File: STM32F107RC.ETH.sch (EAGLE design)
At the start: 28 parts, among them J1 HR911105A, Q1 8MHz, U1 LAN8720A-CP, U2 STM32F107RCT6, X1 CB3LV-3I-74M2500

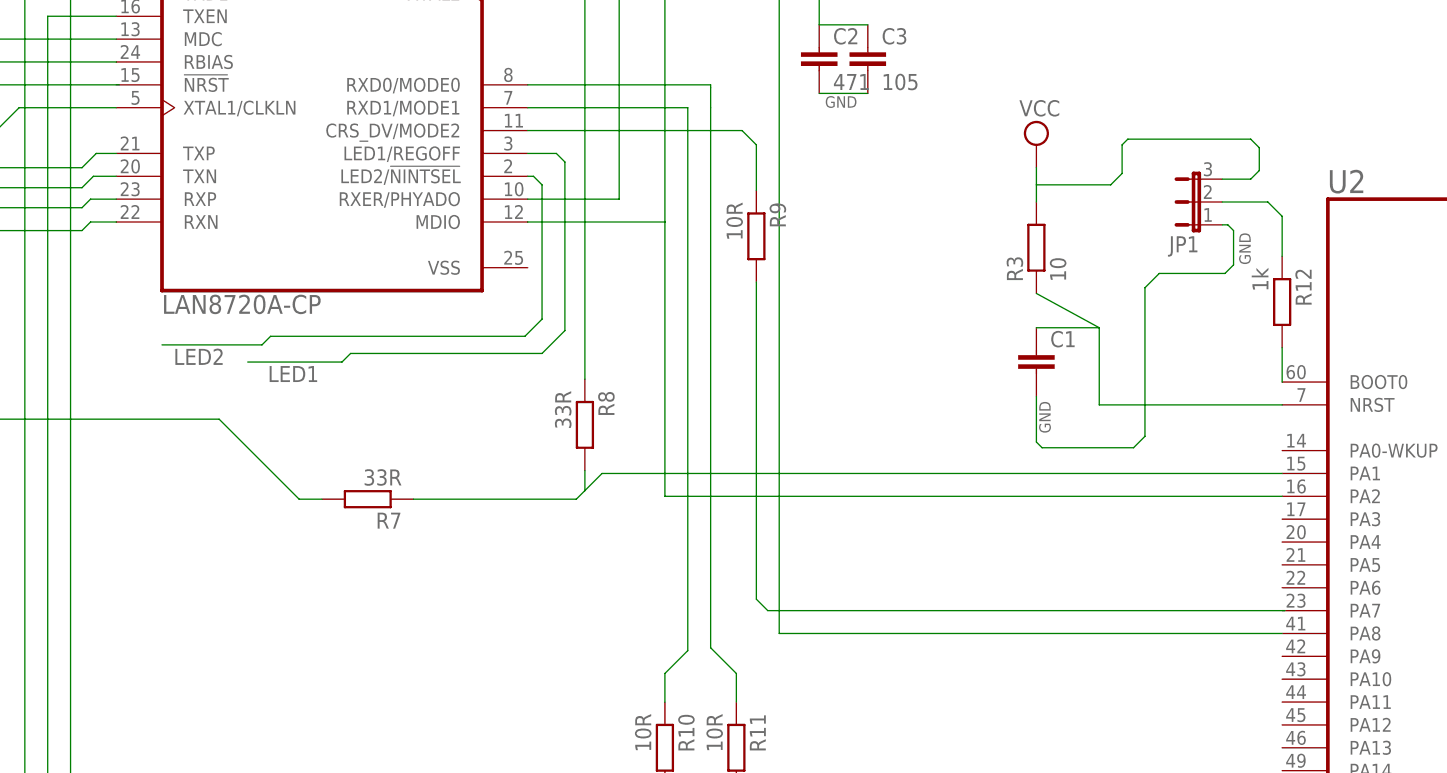
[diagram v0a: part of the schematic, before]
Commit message: Add files via upload
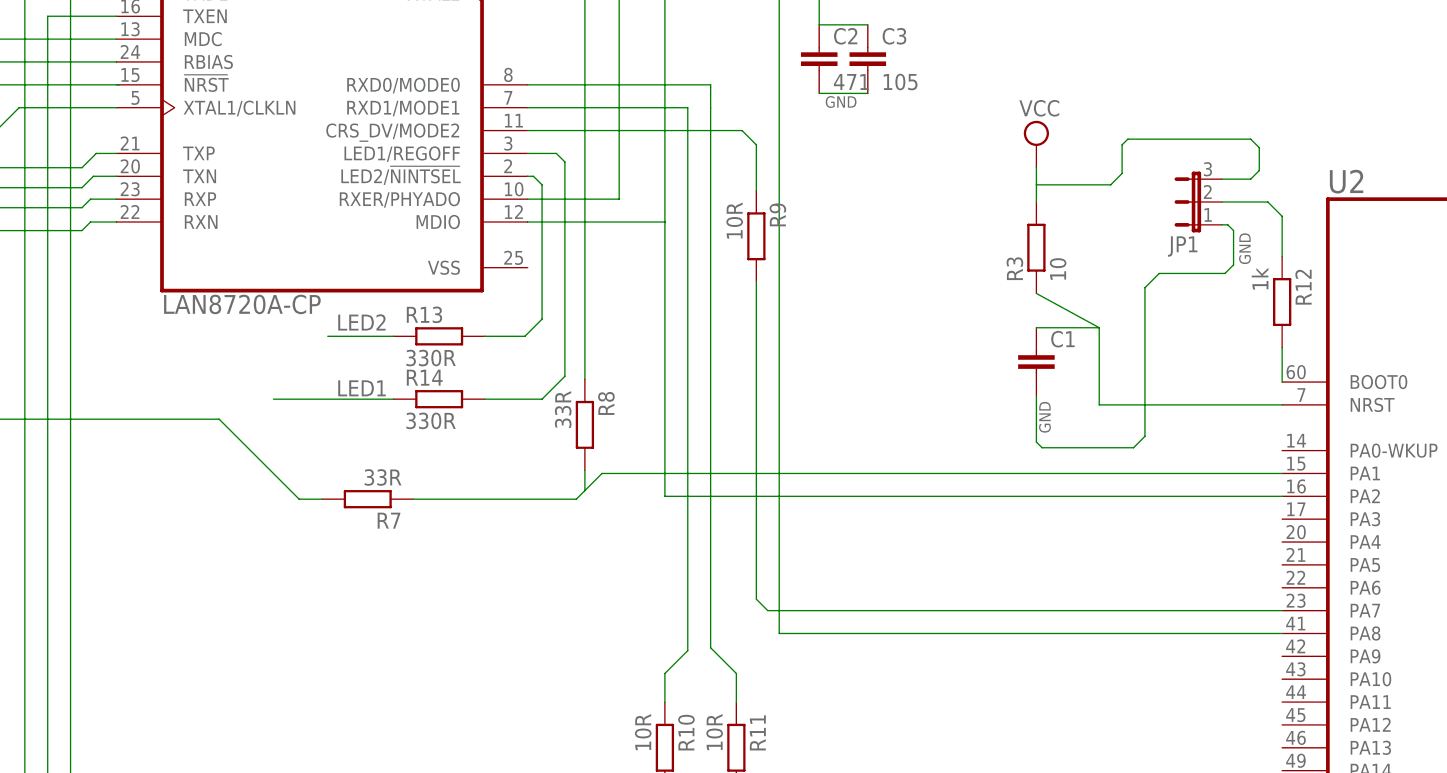
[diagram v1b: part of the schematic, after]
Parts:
- added R13, R14: 330R, resistor:R-EU_0204_7
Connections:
- new net SIG_LED01: R14.2, U1.LED1/REGOFF
- new net SIG_LED02: R13.2, U1.LED2/!NINTSEL!
- net LED1: now also R14.1; no longer U1.LED1/REGOFF
- net LED2: now also R13.1; no longer U1.LED2/!NINTSEL!
- net N$4: now also U2.PA7
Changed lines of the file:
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@@
 <part name="J1" library="HR911105A" deviceset="HR911105A" device=""/>
 <part name="J2" library="SparkFun-Connectors" deviceset="M01" device="OFFSET"/>
+<part name="R13" library="resistor" deviceset="R-EU_" device="0204_7" value="330R"/>
+<part name="R14" library="resistor" deviceset="R-EU_" device="0204_7" value="330R"/>
 </parts>
 <sheets>
@@
 <instance part="J1" gate="G$1" x="-158.115" y="139.3825" rot="R180"/>
 <instance part="J2" gate="G$1" x="17.78" y="198.12" rot="R270"/>
+<instance part="R13" gate="G$1" x="-12.3825" y="124.46"/>
+<instance part="R14" gate="G$1" x="-12.3825" y="117.475"/>
 </instances>
 <busses>
@@
 <net name="N$4" class="0">
 <segment>
-<wire x1="81.5975" y1="93.98" x2="24.13" y2="93.98" width="0.1524" layer="91"/>
+<wire x1="81.28" y1="93.98" x2="24.13" y2="93.98" width="0.1524" layer="91"/>
 <pinref part="R9" gate="G$1" pin="2"/>
 <wire x1="22.86" y1="130.4925" x2="22.86" y2="95.25" width="0.1524" layer="91"/>
 <wire x1="22.86" y1="95.25" x2="24.13" y2="93.98" width="0.1524" layer="91"/>
+<pinref part="U2" gate="A" pin="PA7"/>
 </segment>
 </net>
@@
 <net name="LED2" class="0">
 <segment>
-<pinref part="U1" gate="G$1" pin="LED2/!NINTSEL!"/>
-<wire x1="-2.54" y1="142.24" x2="-1.905" y2="142.24" width="0.1524" layer="91"/>
-<wire x1="-1.905" y1="142.24" x2="-0.9525" y2="141.2875" width="0.1524" layer="91"/>
-<wire x1="-0.9525" y1="141.2875" x2="-0.9525" y2="126.365" width="0.1524" layer="91"/>
-<wire x1="-0.9525" y1="126.365" x2="-2.8575" y2="124.46" width="0.1524" layer="91"/>
-<wire x1="-2.8575" y1="124.46" x2="-31.115" y2="124.46" width="0.1524" layer="91"/>
-<wire x1="-31.115" y1="124.46" x2="-32.0675" y2="123.5075" width="0.1524" layer="91"/>
-<wire x1="-32.0675" y1="123.5075" x2="-43.18" y2="123.5075" width="0.1524" layer="91"/>
-<label x="-41.91" y="121.285" size="1.778" layer="95"/>
-</segment>
-<segment>
 <pinref part="J1" gate="G$1" pin="YC"/>
 <wire x1="-120.015" y1="167.3225" x2="-119.0625" y2="167.3225" width="0.1524" layer="91"/>
@@
 <label x="-118.4275" y="180.975" size="1.778" layer="95" rot="R90"/>
 </segment>
+<segment>
+<pinref part="R13" gate="G$1" pin="1"/>
+<wire x1="-17.4625" y1="124.46" x2="-24.765" y2="124.46" width="0.1524" layer="91"/>
+<label x="-23.8125" y="125.095" size="1.778" layer="95"/>
+</segment>
 </net>
 <net name="LED1" class="0">
-<segment>
-<pinref part="U1" gate="G$1" pin="LED1/REGOFF"/>
-<wire x1="-2.54" y1="144.78" x2="0.635" y2="144.78" width="0.1524" layer="91"/>
-<wire x1="0.635" y1="144.78" x2="1.5875" y2="143.8275" width="0.1524" layer="91"/>
-<wire x1="1.5875" y1="143.8275" x2="1.5875" y2="125.095" width="0.1524" layer="91"/>
-<wire x1="1.5875" y1="125.095" x2="-0.9525" y2="122.555" width="0.1524" layer="91"/>
-<wire x1="-0.9525" y1="122.555" x2="-22.225" y2="122.555" width="0.1524" layer="91"/>
-<wire x1="-22.225" y1="122.555" x2="-23.1775" y2="121.6025" width="0.1524" layer="91"/>
-<wire x1="-23.1775" y1="121.6025" x2="-33.655" y2="121.6025" width="0.1524" layer="91"/>
-<label x="-31.4325" y="119.38" size="1.778" layer="95"/>
-</segment>
 <segment>
 <pinref part="J1" gate="G$1" pin="GC"/>
@@
 <label x="-112.7125" y="181.2925" size="1.778" layer="95" rot="R90"/>
 </segment>
-</net>
+<segment>
+<pinref part="R14" gate="G$1" pin="1"/>
+<wire x1="-17.4625" y1="117.475" x2="-30.7975" y2="117.475" width="0.1524" layer="91"/>
+<label x="-23.8125" y="117.7925" size="1.778" layer="95"/>
+</segment>
+</net>
+<net name="SIG_LED02" class="0">
+<segment>
+<pinref part="U1" gate="G$1" pin="LED2/!NINTSEL!"/>
+<wire x1="-2.54" y1="142.24" x2="-1.905" y2="142.24" width="0.1524" layer="91"/>
+<wire x1="-1.905" y1="142.24" x2="-0.9525" y2="141.2875" width="0.1524" layer="91"/>
+<wire x1="-0.9525" y1="141.2875" x2="-0.9525" y2="126.365" width="0.1524" layer="91"/>
+<wire x1="-0.9525" y1="126.365" x2="-2.8575" y2="124.46" width="0.1524" layer="91"/>
+<pinref part="R13" gate="G$1" pin="2"/>
+<wire x1="-2.8575" y1="124.46" x2="-7.3025" y2="124.46" width="0.1524" layer="91"/>
+</segment>
+</net>
+<net name="SIG_LED01" class="0">
+<segment>
+<pinref part="U1" gate="G$1" pin="LED1/REGOFF"/>
+<wire x1="-2.54" y1="144.78" x2="0.635" y2="144.78" width="0.1524" layer="91"/>
+<wire x1="0.635" y1="144.78" x2="1.5875" y2="143.8275" width="0.1524" layer="91"/>
+<wire x1="1.5875" y1="143.8275" x2="1.5875" y2="120.015" width="0.1524" layer="91"/>
+<wire x1="1.5875" y1="120.015" x2="-0.9525" y2="117.475" width="0.1524" layer="91"/>
+<pinref part="R14" gate="G$1" pin="2"/>
+<wire x1="-0.9525" y1="117.475" x2="-7.3025" y2="117.475" width="0.1524" layer="91"/>
+</segment>
+</net>
